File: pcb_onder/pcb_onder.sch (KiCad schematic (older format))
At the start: 15 parts, among them J1 Conn_01x10_Female

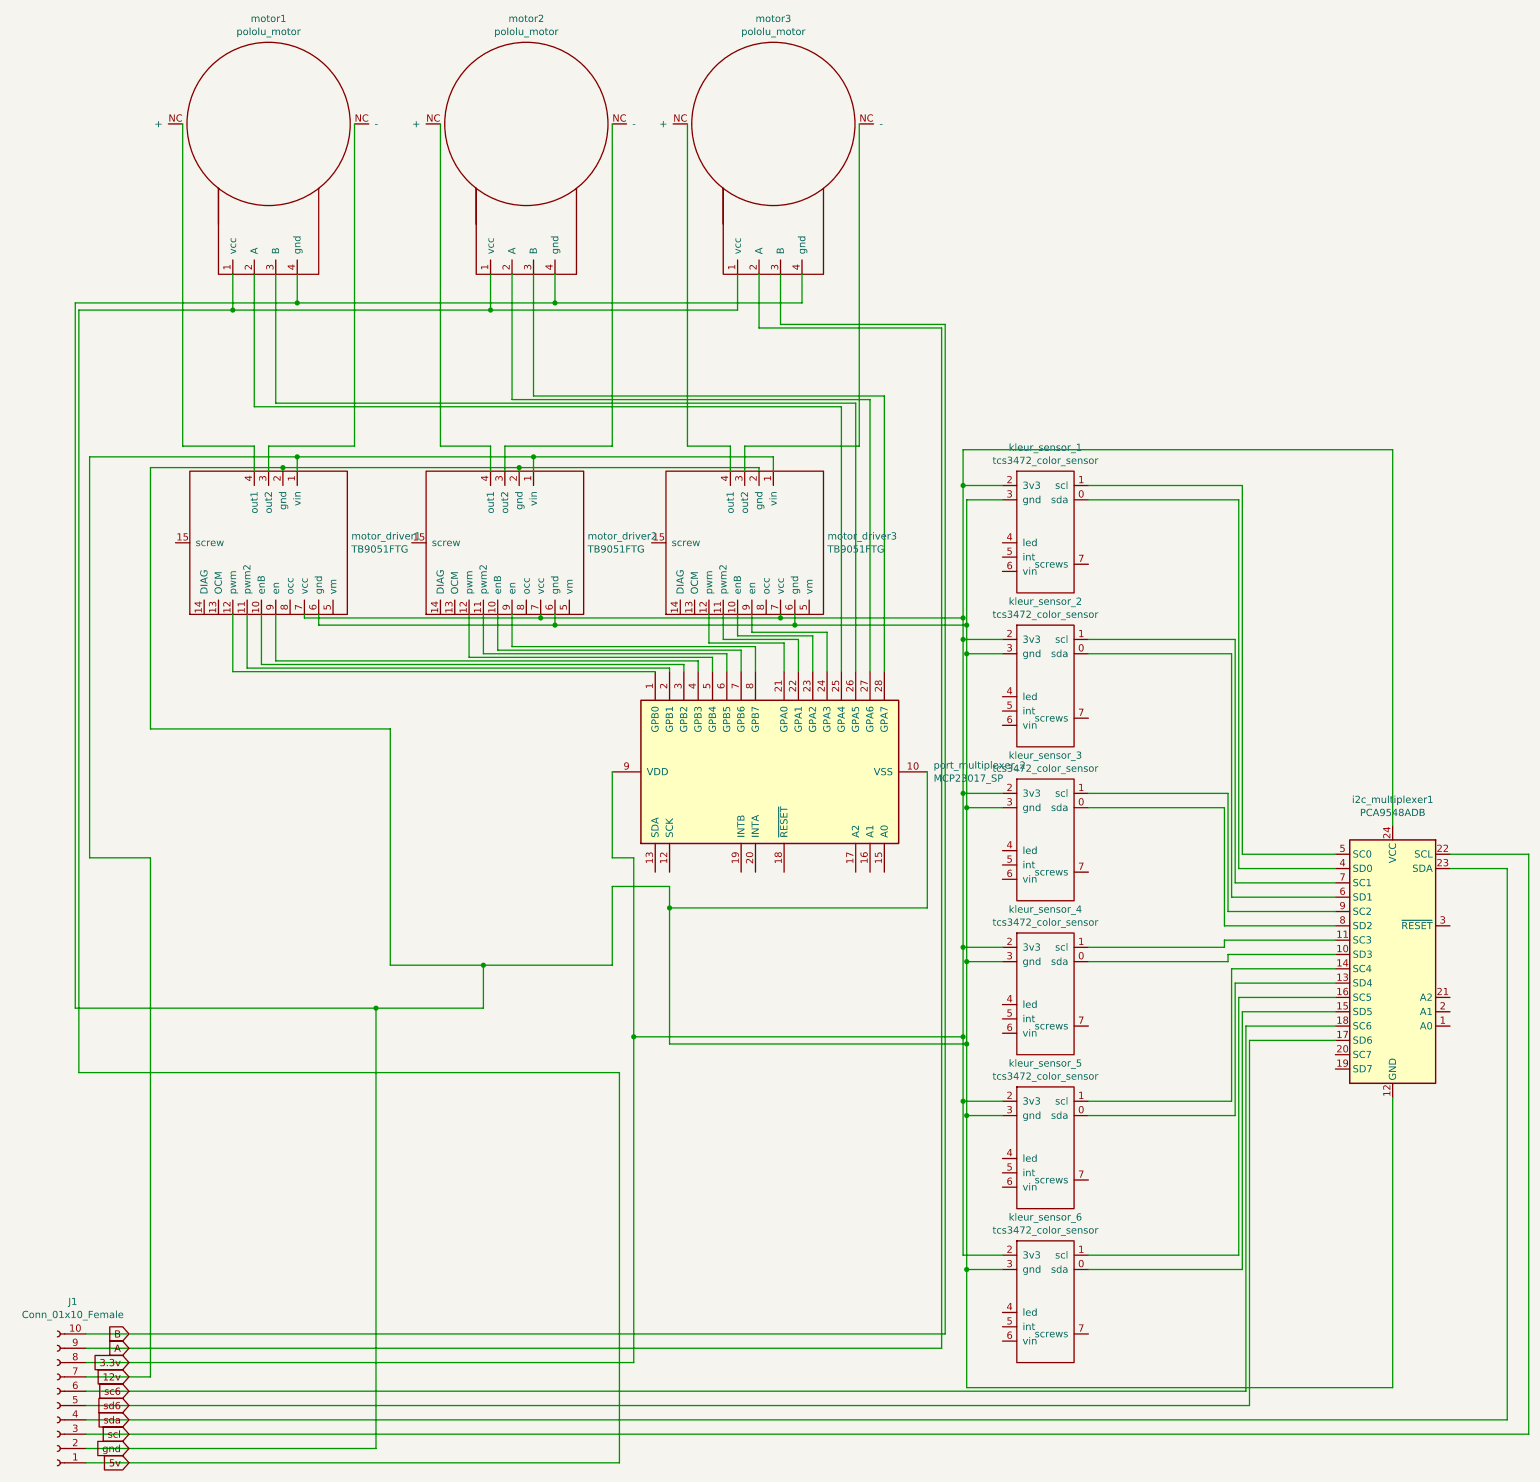
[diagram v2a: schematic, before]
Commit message: i2c
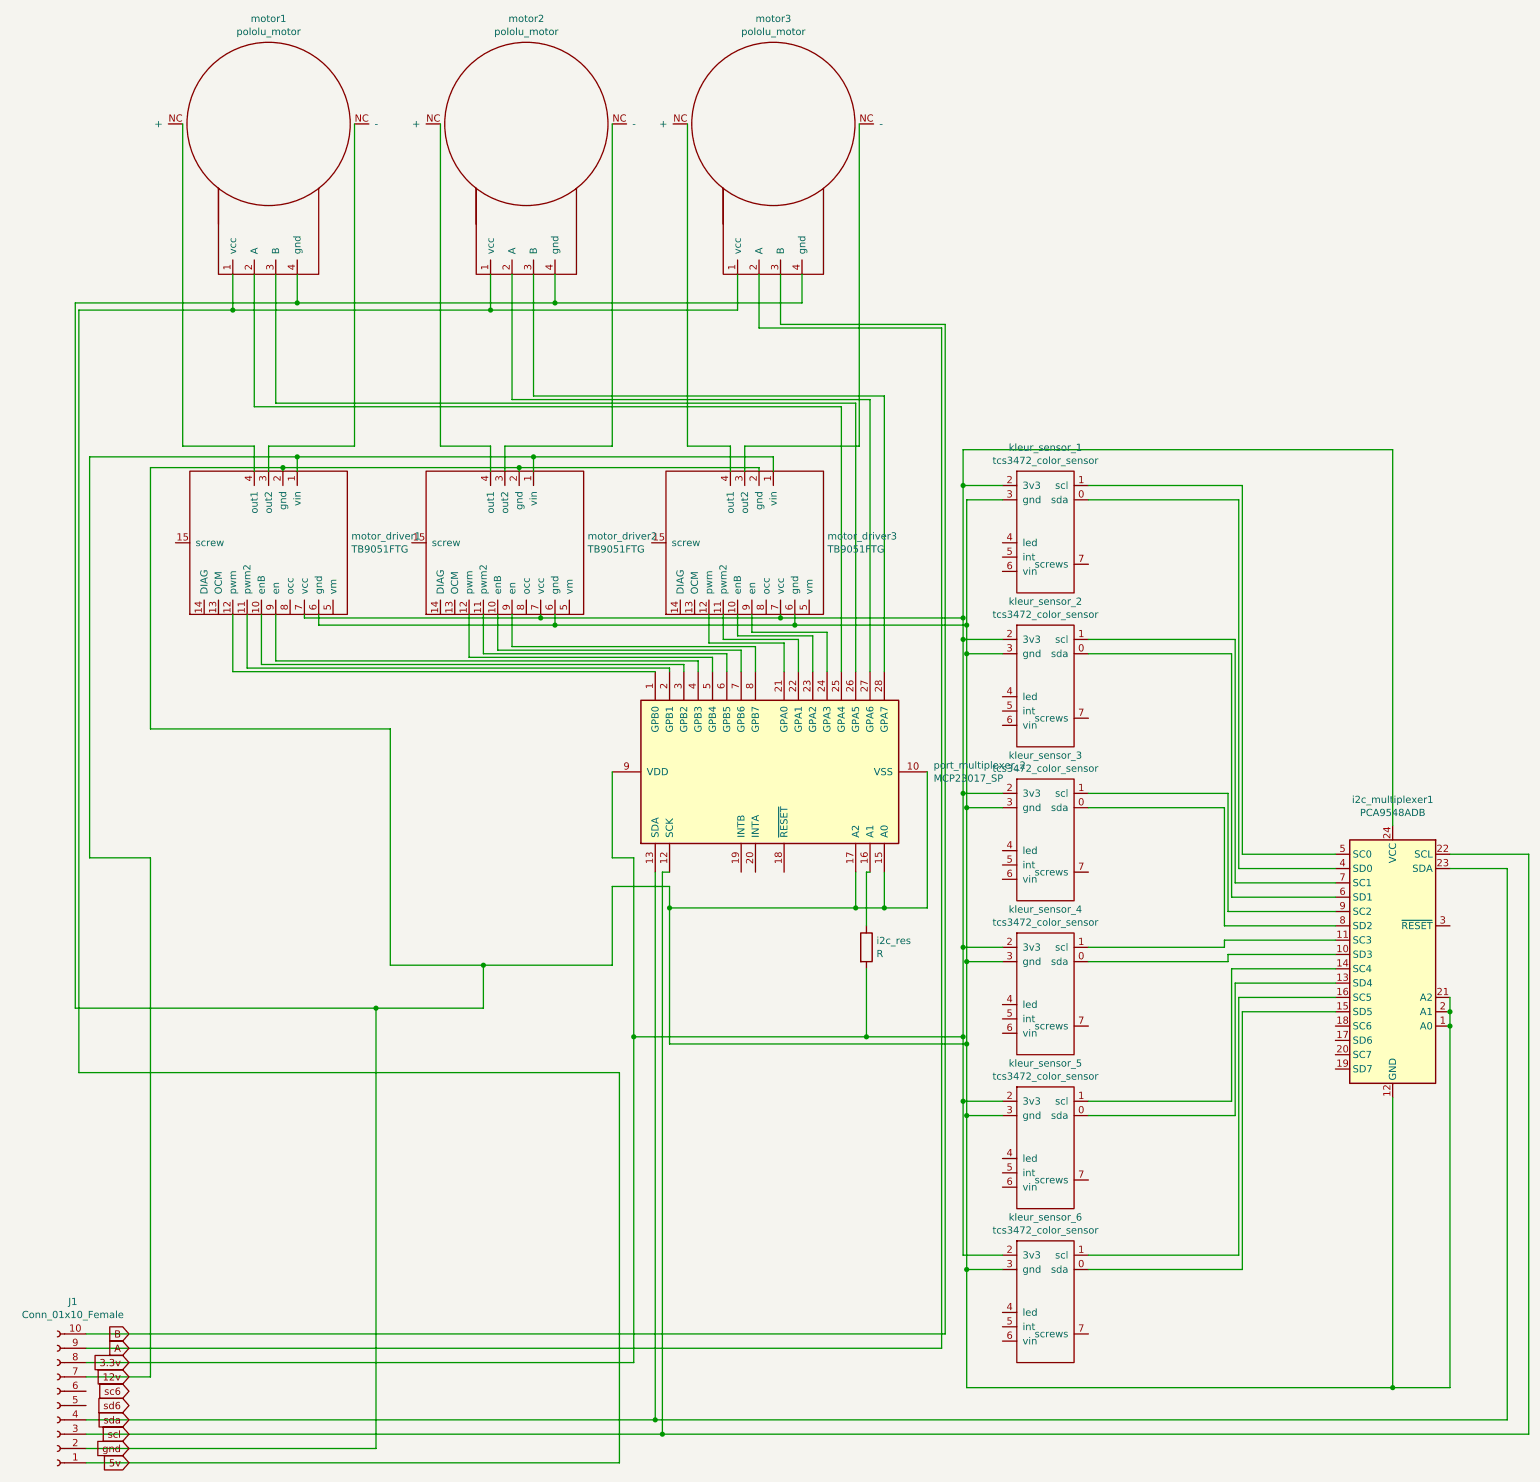
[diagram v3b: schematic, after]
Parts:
- added i2c_res: R, custom:resistor, symbol Device:R
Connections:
- net 3.3v: now also i2c_res.2
- net gnd: now also i2c_multiplexer1.1 (A0), i2c_multiplexer1.2 (A1), i2c_multiplexer1.21 (A2), port_multiplexer_2.15 (A0), port_multiplexer_2.17 (A2)
- net sc6: no longer J1.6 (Pin_6), i2c_multiplexer1.18 (SC6)
- net scl: now also port_multiplexer_2.12 (SCK)
- net sd6: no longer J1.5 (Pin_5), i2c_multiplexer1.17 (SD6)
- net sda: now also port_multiplexer_2.13 (SDA)
- net at port_multiplexer_2.16 (A1): now also i2c_res.1
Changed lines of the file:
@@
 Wire Wire Line
 	9025 7925 9675 7925
-Wire Wire Line
-	9675 8025 9050 8025
-Wire Wire Line
-	9050 8025 9050 10575
-Wire Wire Line
-	9050 10575 950  10575
 Text GLabel 1250 10575 0    50   Input ~ 0
 sc6
-Wire Wire Line
-	950  10675 9075 10675
-Wire Wire Line
-	9075 10675 9075 8125
-Wire Wire Line
-	9075 8125 9675 8125
 Text GLabel 1250 10675 0    50   Input ~ 0
 sd6
@@
 Wire Wire Line
 	11025 6825 11025 10875
-Wire Wire Line
-	11025 10875 950  10875
-Wire Wire Line
-	950  10775 10875 10775
 Text GLabel 1250 10775 0    50   Input ~ 0
 sda
@@
 	6825 6250 6825 7200
 Wire Wire Line
-	6825 7200 5025 7200
+	6825 7200 6525 7200
 Connection ~ 5025 7200
 Wire Wire Line
@@
 	7075 5175 7075 5325
 Wire Wire Line
-	4775 8100 7075 8100
+	4775 8100 6400 8100
 Connection ~ 4775 8100
 Wire Wire Line
@@
 Wire Wire Line
 	3075 5950 3075 7600
+Wire Wire Line
+	6325 6950 6325 7200
+Connection ~ 6325 7200
+Wire Wire Line
+	6325 7200 5025 7200
+Wire Wire Line
+	6525 6950 6525 7200
+Connection ~ 6525 7200
+Wire Wire Line
+	6525 7200 6325 7200
+$Comp
+L Device:R i2c_res
+U 1 1 666C9452
+P 6400 7475
+F 0 "i2c_res" H 6470 7521 50  0000 L CNN
+F 1 "R" H 6470 7430 50  0000 L CNN
+F 2 "custom:resistor" V 6330 7475 50  0001 C CNN
+F 3 "~" H 6400 7475 50  0001 C CNN
+	1    6400 7475
+	1    0    0    -1
+$EndComp
+Wire Wire Line
+	6400 8100 6400 7625
+Connection ~ 6400 8100
+Wire Wire Line
+	6400 8100 7075 8100
+Wire Wire Line
+	6400 7325 6400 6950
+Wire Wire Line
+	6400 6950 6425 6950
+Wire Wire Line
+	4925 6950 4925 10775
+Wire Wire Line
+	950  10775 4925 10775
+Connection ~ 4925 10775
+Wire Wire Line
+	4925 10775 10875 10775
+Wire Wire Line
+	5025 6950 4975 6950
+Wire Wire Line
+	4975 6950 4975 10875
+Wire Wire Line
+	950  10875 4975 10875
+Connection ~ 4975 10875
+Wire Wire Line
+	4975 10875 11025 10875
+Wire Wire Line
+	10475 7825 10475 7925
+Wire Wire Line
+	10475 7925 10475 8025
+Connection ~ 10475 7925
+Wire Wire Line
+	10475 8025 10475 10550
+Wire Wire Line
+	10475 10550 10075 10550
+Connection ~ 10475 8025
+Connection ~ 10075 10550
 $EndSCHEMATC
